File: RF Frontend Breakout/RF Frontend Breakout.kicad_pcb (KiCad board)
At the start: 2 copper layers, 122.5 x 83 mm, 54 parts, among them IC1 QPC1022SR, IC2 GRF5504, IC3 LHA-13LN+, IC4 QPC1022SR, J3 Conn_Coaxial, J4 Conn_01x02, J5 Conn_01x02, J6 Conn_Coaxial

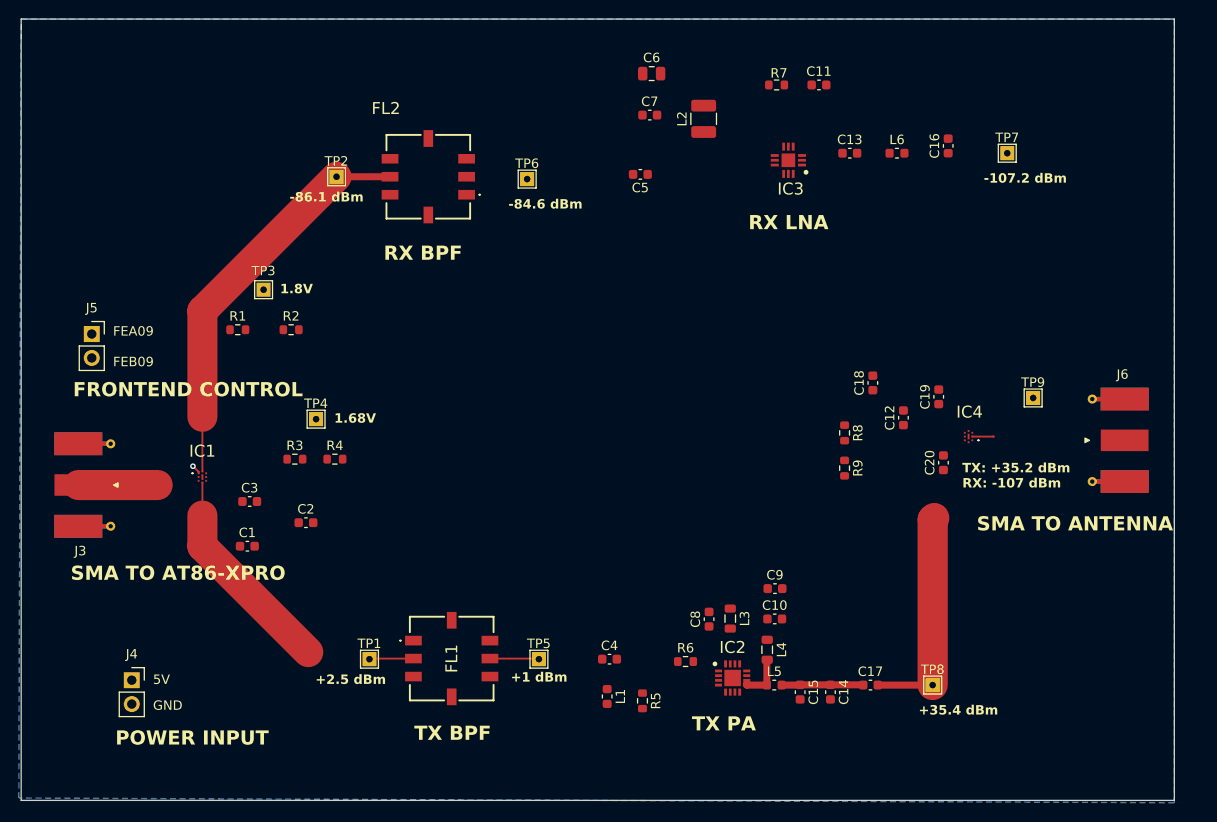
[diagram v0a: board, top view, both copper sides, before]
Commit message: test
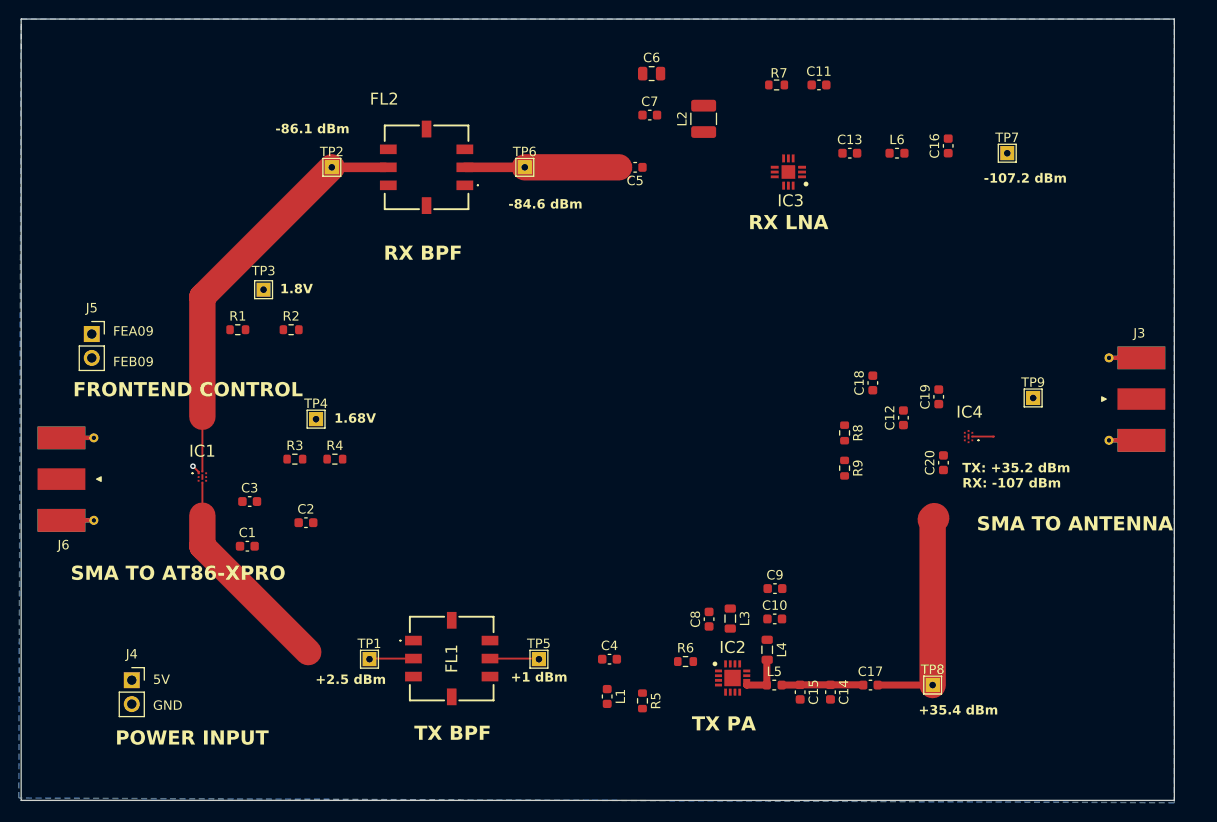
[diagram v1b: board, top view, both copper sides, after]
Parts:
- moved J3 109.9 mm to (193.3, 112.1), turned to 180 degrees
- moved J6 109.6 mm to (82.0, 120.6), turned to 0 degrees
- moved TP6 1.27 mm to (129.5, 87.5)
- moved IC3 1.25 mm to (157.5, 88.0)
- moved TP2 1.12 mm to (109.0, 87.5)
- moved FL2 1.02 mm to (119.1, 87.5)
- moved C5 0.93 mm to (141.2, 87.5)
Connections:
- C20 pad 1: Net-(J6-Ext) -> Net-(J6-In)
- J6 pad 1: GND -> Net-(J6-In)
- J6 pad 2: Net-(J6-Ext) -> GND
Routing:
- net Net-(FL2-RF_IN): track 0.00 -> 16.7 mm
- net Net-(IC4-ANT): track 10.7 -> 2.31 mm
- net Net-(FL2-RF_OUT): track 42.9 -> 43.7 mm

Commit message: finished pcb
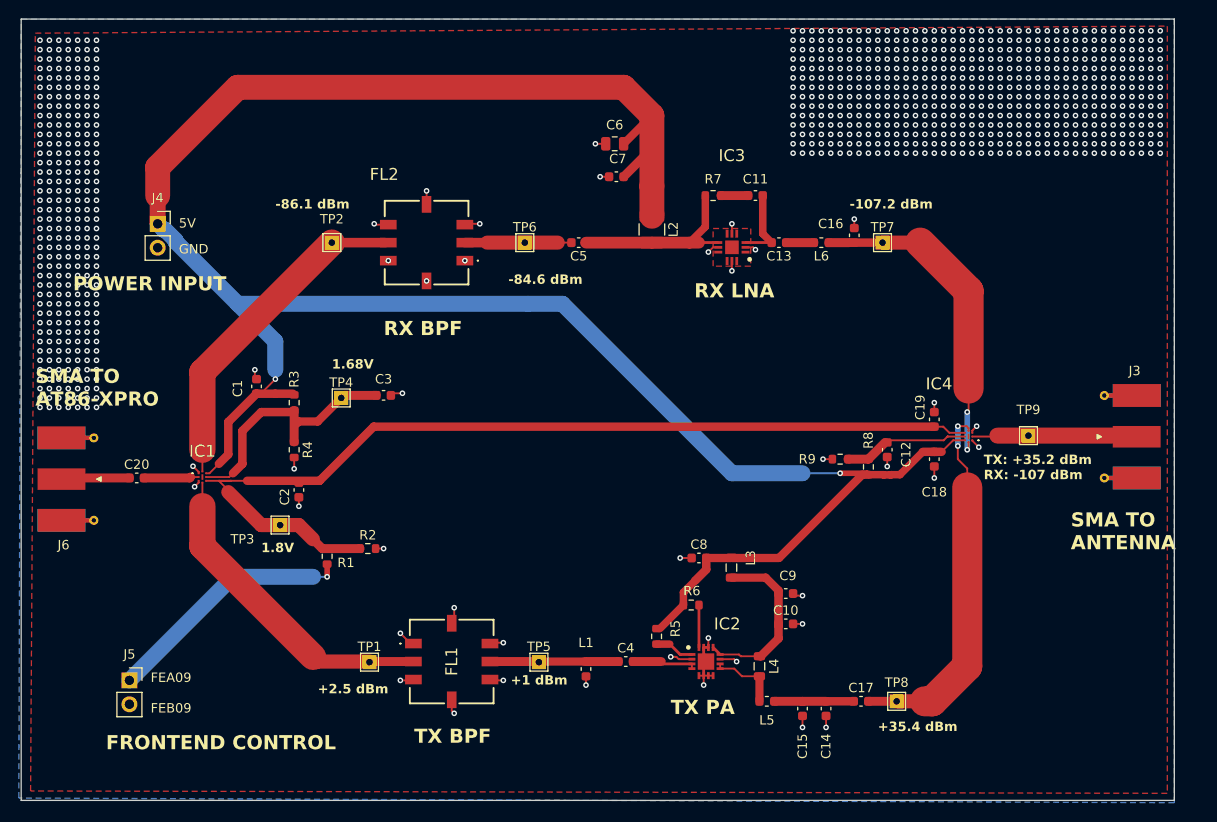
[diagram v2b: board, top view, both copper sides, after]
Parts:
- moved C20 85.7 mm to (88.3, 120.5), turned to 0 degrees
- moved J4 48.6 mm to (90.5, 93.5)
- moved J5 37.0 mm to (87.5, 142.0)
- moved R1 25.9 mm to (108.5, 128.8), turned to 90 degrees
- moved TP3 25.1 mm to (103.5, 125.5)
- moved R2 24.6 mm to (112.8, 128.0)
- moved C3 18.2 mm to (114.5, 111.7)
- moved C1 17.0 mm to (101.0, 110.8), turned to 90 degrees
- moved TP7 16.3 mm to (167.5, 95.5)
- moved C16 13.8 mm to (164.5, 94.7)
- moved C11 13.6 mm to (154.0, 90.5), turned to 180 degrees
- moved R7 13.6 mm to (149.5, 90.5)
- moved L2 13.0 mm to (143.0, 94.1), turned to -90 degrees
- moved L6 12.4 mm to (161.0, 95.5), turned to 180 degrees
- moved C13 12.1 mm to (156.5, 95.5), turned to 180 degrees
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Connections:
- J4 pad 1: Net-(J4-Pin_1) -> +5V
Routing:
- net +5V: track 0.00 -> 251.2 mm, vias 0 -> 2
- net Net-(IC1-CTRL): track 0.00 -> 102.6 mm
- net GND: track 1.00 -> 52.7 mm, vias 1 -> 882
- net Net-(IC4-RF2): track 0.00 -> 34.8 mm, vias 0 -> 2
- net Net-(IC1-EN): track 0.00 -> 27.8 mm
- net /FEA09: track 0.00 -> 26.9 mm, vias 0 -> 1
- net Net-(IC3-RF-OUT&DC-IN): track 0.00 -> 19.7 mm
- net Net-(IC2-BIAS): track 0.00 -> 19.2 mm
- net Net-(IC4-ANT): track 2.31 -> 21.5 mm
- net Net-(IC4-RF1): track 23.7 -> 40.3 mm, vias 0 -> 2
- net Net-(IC4-EN): track 0.00 -> 13.4 mm
- net Net-(FL1-RF_OUT): track 5.23 -> 13.7 mm
- net Net-(IC3-RF-IN): track 0.00 -> 8.19 mm
- net Net-(FL2-RF_OUT): track 43.7 -> 35.7 mm
- net Net-(J6-In): track 0.00 -> 7.27 mm
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- added copper zone on F.Cu, net GND
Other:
- board text added: "+5V"

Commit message: small changes after larry meeting will populate his changes later
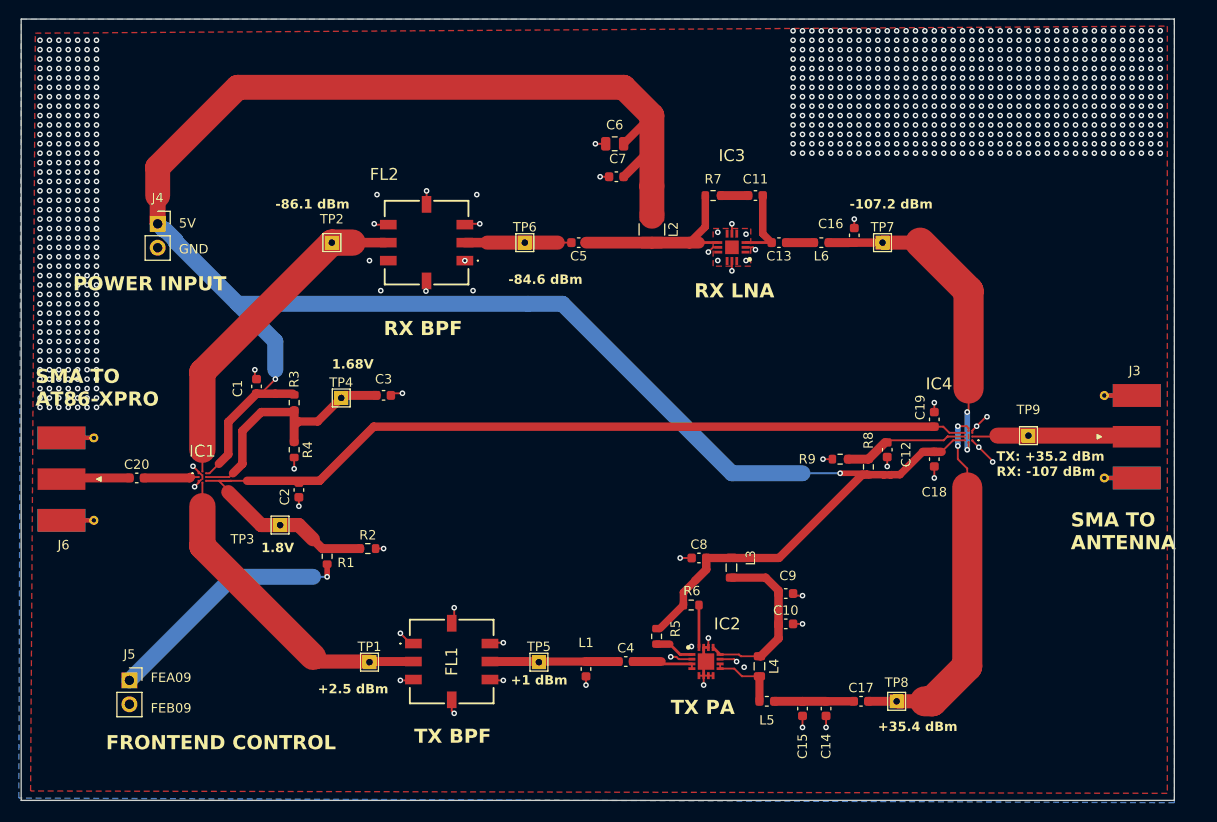
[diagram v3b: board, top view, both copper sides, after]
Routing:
- net GND: track 52.7 -> 56.9 mm, vias 882 -> 894
- net Net-(FL2-RF_OUT): track 35.7 -> 37.9 mm
